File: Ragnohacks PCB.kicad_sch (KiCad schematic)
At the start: 35 parts, among them J1 Conn_01x02, J2 Conn_01x18, J3 Conn_01x18, J4 USB_A, SW1 SW_Push, U1 RP2040, U2 W25Q128JVS, U3 LD1117S33TR_SOT223, U4 USBLC6-2P6, Y1 12MHz

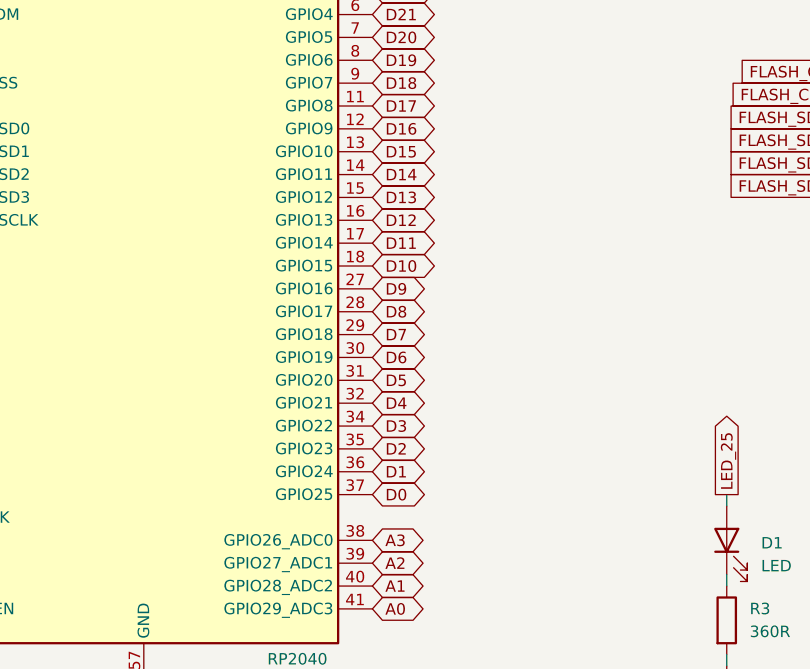
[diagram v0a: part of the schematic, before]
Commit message: Finish tracing
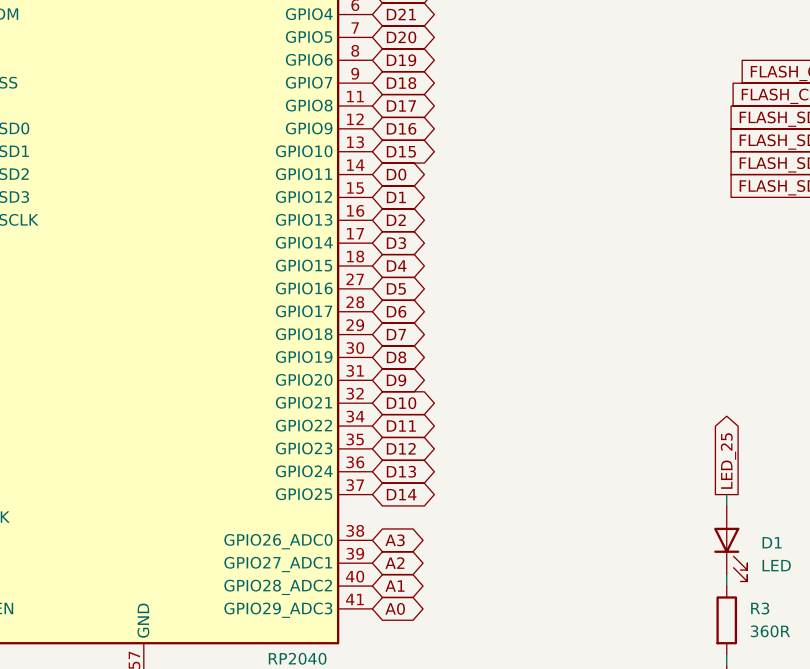
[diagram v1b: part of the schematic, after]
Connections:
- net D0: now also U1.14 (GPIO11); no longer U1.37 (GPIO25)
- net D1: now also U1.15 (GPIO12); no longer U1.36 (GPIO24)
- net D10: now also U1.32 (GPIO21); no longer U1.18 (GPIO15)
- net D11: now also U1.34 (GPIO22); no longer U1.17 (GPIO14)
- net D12: now also U1.35 (GPIO23); no longer U1.16 (GPIO13)
- net D13: now also U1.36 (GPIO24); no longer U1.15 (GPIO12)
- net D14: now also U1.37 (GPIO25); no longer U1.14 (GPIO11)
- net D2: now also U1.16 (GPIO13); no longer U1.35 (GPIO23)
- net D3: now also U1.17 (GPIO14); no longer U1.34 (GPIO22)
- net D4: now also U1.18 (GPIO15); no longer U1.32 (GPIO21)
- net D5: now also U1.27 (GPIO16); no longer U1.31 (GPIO20)
- net D6: now also U1.28 (GPIO17); no longer U1.30 (GPIO19)
- net D8: now also U1.30 (GPIO19); no longer U1.28 (GPIO17)
- net D9: now also U1.31 (GPIO20); no longer U1.27 (GPIO16)
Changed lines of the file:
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@@
 	(global_label "D1"
 		(shape bidirectional)
-		(at 104.14 110.49 0)
-		(fields_autoplaced yes)
-		(effects
-			(font
-				(size 1.27 1.27)
-			)
-			(justify left)
-		)
-		(property "Intersheetrefs" "${INTERSHEET_REFS}"
-			(at 110.716 110.49 0)
+		(at 104.14 80.01 0)
+		(fields_autoplaced yes)
+		(effects
+			(font
+				(size 1.27 1.27)
+			)
+			(justify left)
+		)
+		(property "Intersheetrefs" "${INTERSHEET_REFS}"
+			(at 110.716 80.01 0)
 			(effects
 				(font
@@
 	(global_label "D10"
 		(shape bidirectional)
-		(at 104.14 87.63 0)
-		(fields_autoplaced yes)
-		(effects
-			(font
-				(size 1.27 1.27)
-			)
-			(justify left)
-		)
-		(property "Intersheetrefs" "${INTERSHEET_REFS}"
-			(at 111.9255 87.63 0)
+		(at 104.14 102.87 0)
+		(fields_autoplaced yes)
+		(effects
+			(font
+				(size 1.27 1.27)
+			)
+			(justify left)
+		)
+		(property "Intersheetrefs" "${INTERSHEET_REFS}"
+			(at 111.9255 102.87 0)
 			(effects
 				(font
@@
 	(global_label "D0"
 		(shape bidirectional)
-		(at 104.14 113.03 0)
-		(fields_autoplaced yes)
-		(effects
-			(font
-				(size 1.27 1.27)
-			)
-			(justify left)
-		)
-		(property "Intersheetrefs" "${INTERSHEET_REFS}"
-			(at 110.716 113.03 0)
+		(at 104.14 77.47 0)
+		(fields_autoplaced yes)
+		(effects
+			(font
+				(size 1.27 1.27)
+			)
+			(justify left)
+		)
+		(property "Intersheetrefs" "${INTERSHEET_REFS}"
+			(at 110.716 77.47 0)
 			(effects
 				(font
@@
 	(global_label "D4"
 		(shape bidirectional)
-		(at 104.14 102.87 0)
-		(fields_autoplaced yes)
-		(effects
-			(font
-				(size 1.27 1.27)
-			)
-			(justify left)
-		)
-		(property "Intersheetrefs" "${INTERSHEET_REFS}"
-			(at 110.716 102.87 0)
+		(at 104.14 87.63 0)
+		(fields_autoplaced yes)
+		(effects
+			(font
+				(size 1.27 1.27)
+			)
+			(justify left)
+		)
+		(property "Intersheetrefs" "${INTERSHEET_REFS}"
+			(at 110.716 87.63 0)
 			(effects
 				(font
@@
 	(global_label "D8"
 		(shape bidirectional)
-		(at 104.14 92.71 0)
-		(fields_autoplaced yes)
-		(effects
-			(font
-				(size 1.27 1.27)
-			)
-			(justify left)
-		)
-		(property "Intersheetrefs" "${INTERSHEET_REFS}"
-			(at 110.716 92.71 0)
+		(at 104.14 97.79 0)
+		(fields_autoplaced yes)
+		(effects
+			(font
+				(size 1.27 1.27)
+			)
+			(justify left)
+		)
+		(property "Intersheetrefs" "${INTERSHEET_REFS}"
+			(at 110.716 97.79 0)
 			(effects
 				(font
@@
 	(global_label "D5"
 		(shape bidirectional)
-		(at 104.14 100.33 0)
-		(fields_autoplaced yes)
-		(effects
-			(font
-				(size 1.27 1.27)
-			)
-			(justify left)
-		)
-		(property "Intersheetrefs" "${INTERSHEET_REFS}"
-			(at 110.716 100.33 0)
+		(at 104.14 90.17 0)
+		(fields_autoplaced yes)
+		(effects
+			(font
+				(size 1.27 1.27)
+			)
+			(justify left)
+		)
+		(property "Intersheetrefs" "${INTERSHEET_REFS}"
+			(at 110.716 90.17 0)
 			(effects
 				(font
@@
 	(global_label "D6"
 		(shape bidirectional)
-		(at 104.14 97.79 0)
-		(fields_autoplaced yes)
-		(effects
-			(font
-				(size 1.27 1.27)
-			)
-			(justify left)
-		)
-		(property "Intersheetrefs" "${INTERSHEET_REFS}"
-			(at 110.716 97.79 0)
+		(at 104.14 92.71 0)
+		(fields_autoplaced yes)
+		(effects
+			(font
+				(size 1.27 1.27)
+			)
+			(justify left)
+		)
+		(property "Intersheetrefs" "${INTERSHEET_REFS}"
+			(at 110.716 92.71 0)
 			(effects
 				(font
@@
 	(global_label "D2"
 		(shape bidirectional)
-		(at 104.14 107.95 0)
-		(fields_autoplaced yes)
-		(effects
-			(font
-				(size 1.27 1.27)
-			)
-			(justify left)
-		)
-		(property "Intersheetrefs" "${INTERSHEET_REFS}"
-			(at 110.716 107.95 0)
+		(at 104.14 82.55 0)
+		(fields_autoplaced yes)
+		(effects
+			(font
+				(size 1.27 1.27)
+			)
+			(justify left)
+		)
+		(property "Intersheetrefs" "${INTERSHEET_REFS}"
+			(at 110.716 82.55 0)
 			(effects
 				(font
@@
 	(global_label "D13"
 		(shape bidirectional)
-		(at 104.14 80.01 0)
-		(fields_autoplaced yes)
-		(effects
-			(font
-				(size 1.27 1.27)
-			)
-			(justify left)
-		)
-		(property "Intersheetrefs" "${INTERSHEET_REFS}"
-			(at 111.9255 80.01 0)
+		(at 104.14 110.49 0)
+		(fields_autoplaced yes)
+		(effects
+			(font
+				(size 1.27 1.27)
+			)
+			(justify left)
+		)
+		(property "Intersheetrefs" "${INTERSHEET_REFS}"
+			(at 111.9255 110.49 0)
 			(effects
 				(font
@@
 	(global_label "D14"
 		(shape bidirectional)
-		(at 104.14 77.47 0)
-		(fields_autoplaced yes)
-		(effects
-			(font
-				(size 1.27 1.27)
-			)
-			(justify left)
-		)
-		(property "Intersheetrefs" "${INTERSHEET_REFS}"
-			(at 111.9255 77.47 0)
+		(at 104.14 113.03 0)
+		(fields_autoplaced yes)
+		(effects
+			(font
+				(size 1.27 1.27)
+			)
+			(justify left)
+		)
+		(property "Intersheetrefs" "${INTERSHEET_REFS}"
+			(at 111.9255 113.03 0)
 			(effects
 				(font
@@
 	(global_label "D3"
 		(shape bidirectional)
-		(at 104.14 105.41 0)
-		(fields_autoplaced yes)
-		(effects
-			(font
-				(size 1.27 1.27)
-			)
-			(justify left)
-		)
-		(property "Intersheetrefs" "${INTERSHEET_REFS}"
-			(at 110.716 105.41 0)
+		(at 104.14 85.09 0)
+		(fields_autoplaced yes)
+		(effects
+			(font
+				(size 1.27 1.27)
+			)
+			(justify left)
+		)
+		(property "Intersheetrefs" "${INTERSHEET_REFS}"
+			(at 110.716 85.09 0)
 			(effects
 				(font
@@
 	(global_label "D9"
 		(shape bidirectional)
-		(at 104.14 90.17 0)
-		(fields_autoplaced yes)
-		(effects
-			(font
-				(size 1.27 1.27)
-			)
-			(justify left)
-		)
-		(property "Intersheetrefs" "${INTERSHEET_REFS}"
-			(at 110.716 90.17 0)
+		(at 104.14 100.33 0)
+		(fields_autoplaced yes)
+		(effects
+			(font
+				(size 1.27 1.27)
+			)
+			(justify left)
+		)
+		(property "Intersheetrefs" "${INTERSHEET_REFS}"
+			(at 110.716 100.33 0)
 			(effects
 				(font
@@
 	(global_label "D11"
 		(shape bidirectional)
-		(at 104.14 85.09 0)
-		(fields_autoplaced yes)
-		(effects
-			(font
-				(size 1.27 1.27)
-			)
-			(justify left)
-		)
-		(property "Intersheetrefs" "${INTERSHEET_REFS}"
-			(at 111.9255 85.09 0)
+		(at 104.14 105.41 0)
+		(fields_autoplaced yes)
+		(effects
+			(font
+				(size 1.27 1.27)
+			)
+			(justify left)
+		)
+		(property "Intersheetrefs" "${INTERSHEET_REFS}"
+			(at 111.9255 105.41 0)
 			(effects
 				(font
@@
 	(global_label "D12"
 		(shape bidirectional)
-		(at 104.14 82.55 0)
-		(fields_autoplaced yes)
-		(effects
-			(font
-				(size 1.27 1.27)
-			)
-			(justify left)
-		)
-		(property "Intersheetrefs" "${INTERSHEET_REFS}"
-			(at 111.9255 82.55 0)
-			(effects
-				(font
+		(at 104.14 107.95 0)
+		(fields_autoplaced yes)
+		(effects
+			(font
+				(size 1.27 1.27)
+			)
+			(justify left)
+		)
+		(property "Intersheetrefs" "${INTERSHEET_REFS}"
+			(at 111.9255 107.95 0)
+			(effects
+				(font

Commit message: The finishing touches
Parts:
- J4: footprint Connector_USB:USB_A_Molex_48037-2200_Horizontal -> Connector_USB:USB_A_Keystone_931_Horizontal
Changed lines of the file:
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@@
 			)
 		)
-		(property "Footprint" "Connector_USB:USB_A_Molex_48037-2200_Horizontal"
+		(property "Footprint" "Connector_USB:USB_A_Keystone_931_Horizontal"
 			(at 40.64 163.83 0)
 			(effects
